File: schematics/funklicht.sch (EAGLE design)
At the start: 23 parts, among them IC2 5V, SW1 push, SW2 push, SW3 push, SW4 push

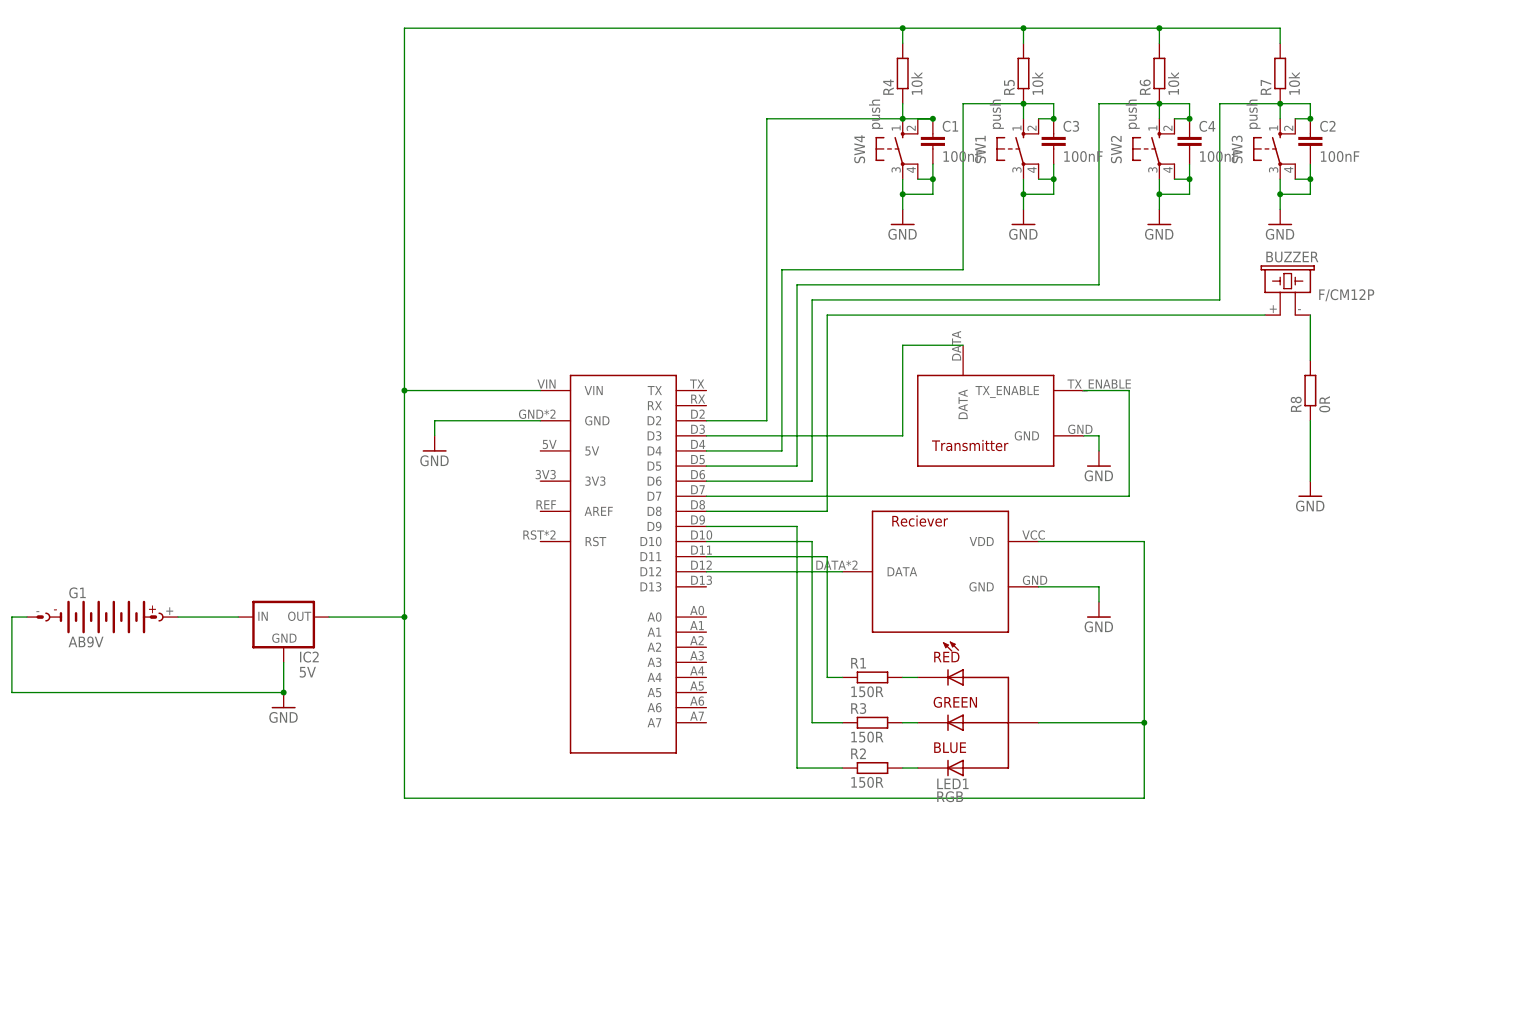
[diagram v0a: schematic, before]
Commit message: schematics done
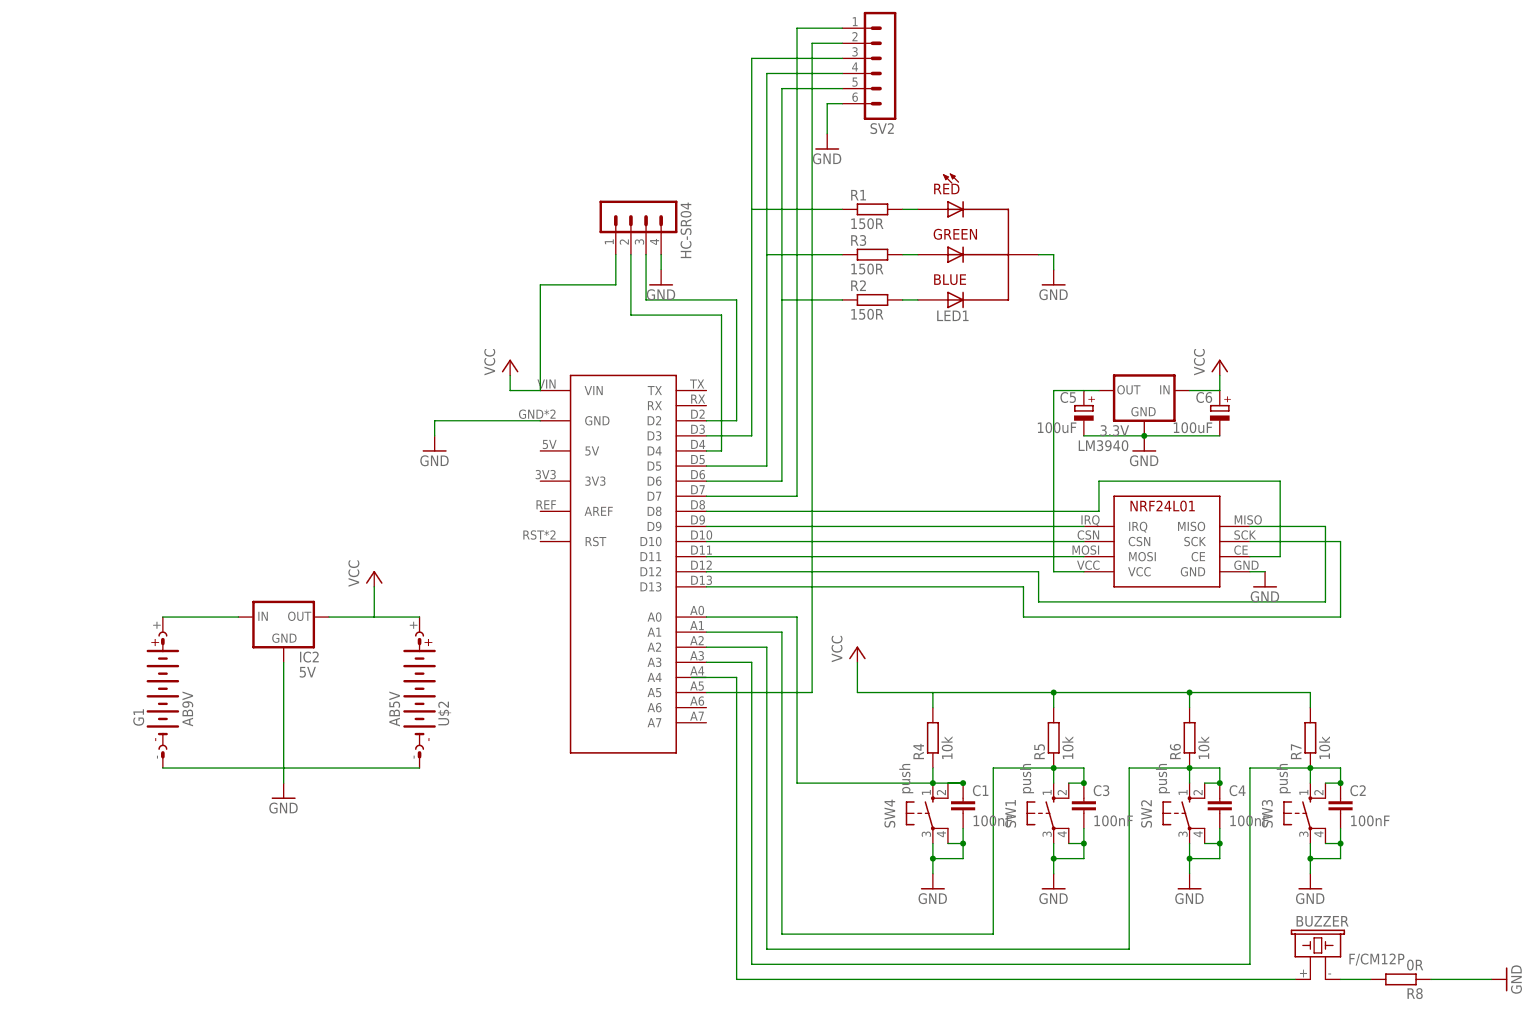
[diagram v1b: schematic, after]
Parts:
- removed U$3: TRANSMITTER, funkmodule:TRANSMITTER
- added 3.3V: LM3940, voltage_regulator:LM3940
- added C5, C6: 100uF, rcl:CPOL-EUTT2D6
- added HC-SR04: (no value), con-lstb:MA04-1
- added SV2: (no value), con-lstb:MA06-1
- added U$4: NRF24L01, funkmodule:NRF24L01
- C1, C2, C3, C4: device rcl:C-EU050-025X075 -> rcl:C-EU025-024X044
- LED1: value RGB -> (none)
- U$2: value RECIEVER -> AB5V; device funkmodule:RECIEVER -> power_supply:AB5V
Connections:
- removed net TX_ENABLE: U$1.D7, U$3.TX_ENABLE
- removed net VDD: IC2.OUT, LED1.VCC, R4.2, R5.2, R6.2, R7.2, U$1.VIN, U$2.VDD
- new net N$10: U$1.D8, U$4.CE
- new net N$11: R3.1, SV2.4, U$1.D5
- new net N$12: R1.1, SV2.3, U$1.D3
- new net N$13: HC-SR04.3, U$1.D2
- new net N$14: HC-SR04.2, U$1.D4
- new net N$21: SV2.1, U$1.D7
- new net N$22: SV2.2, U$1.A5
- new net N$8: U$1.D11, U$4.MOSI
- new net N$9: U$1.D10, U$4.CSN
- new net VCC: 3.3V.IN, C6.+, HC-SR04.1, IC2.OUT, R4.2, R5.2, R6.2, R7.2, U$1.VIN, U$2.+
- net GND: now also 3.3V.GND, C5.-, C6.-, HC-SR04.4, LED1.GND, SV2.6, U$2.-, U$4.GND; no longer U$2.GND, U$3.GND
- net N$1: now also U$1.A0; no longer U$1.D2
- net N$15: now also U$1.A1; no longer U$1.D4
- net N$16: now also U$1.A2; no longer U$1.D5
- net N$17: now also U$1.A3; no longer U$1.D6
- net N$18: no longer U$1.D8
- net N$2: now also R2.1, SV2.5, U$1.D6; no longer U$1.D3, U$3.DATA
- net N$3: now also U$4.MISO; no longer U$2.DATA
- net N$4: now also 3.3V.OUT, C5.+, U$4.VCC; no longer R1.1, U$1.D11
- net N$5: now also U$1.D9, U$4.IRQ; no longer R3.1, U$1.D10
- net N$6: now also U$1.D13, U$4.SCK; no longer R2.1, U$1.D9
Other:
- moved on the sheet: BUZZER, C1, C2, C3, C4, G1, LED1, R1, R2, R3, R4, R5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
